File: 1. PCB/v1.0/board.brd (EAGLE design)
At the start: 69.5 x 114 mm, 2 parts

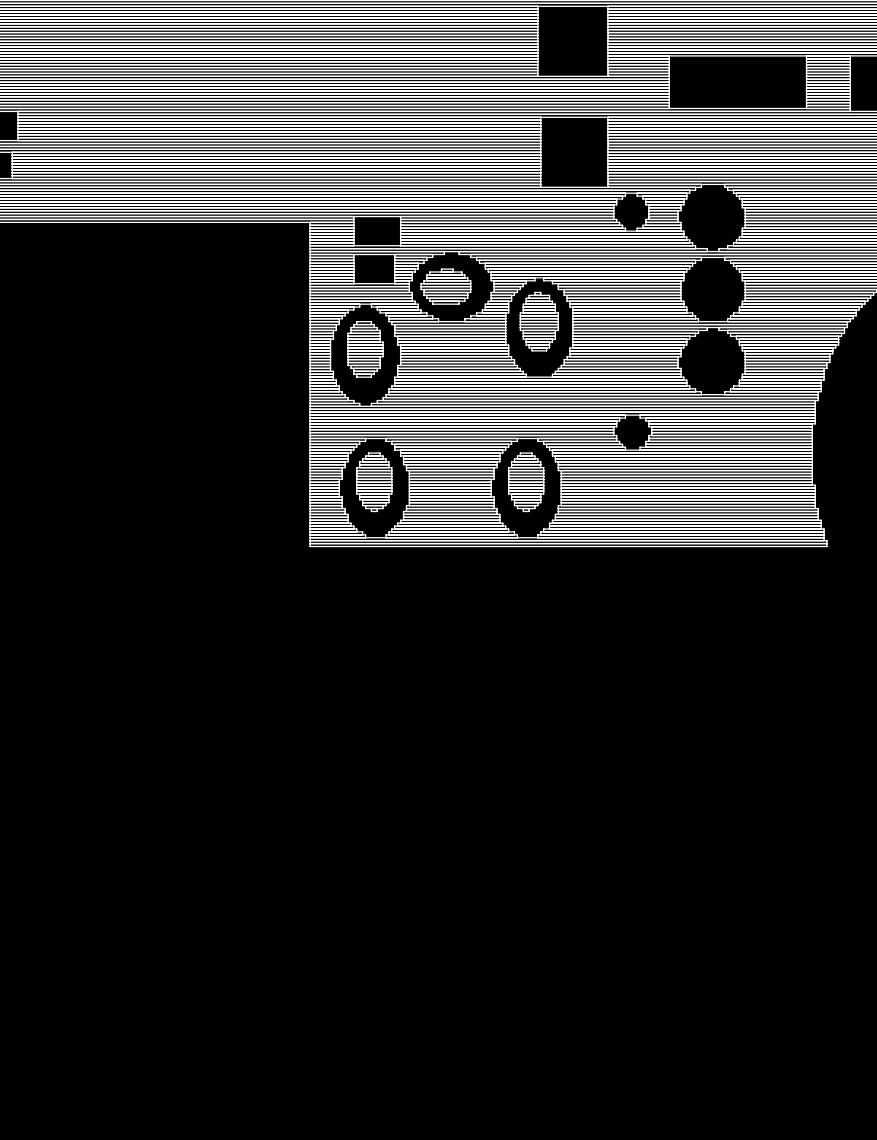
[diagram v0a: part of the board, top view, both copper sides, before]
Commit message: no message
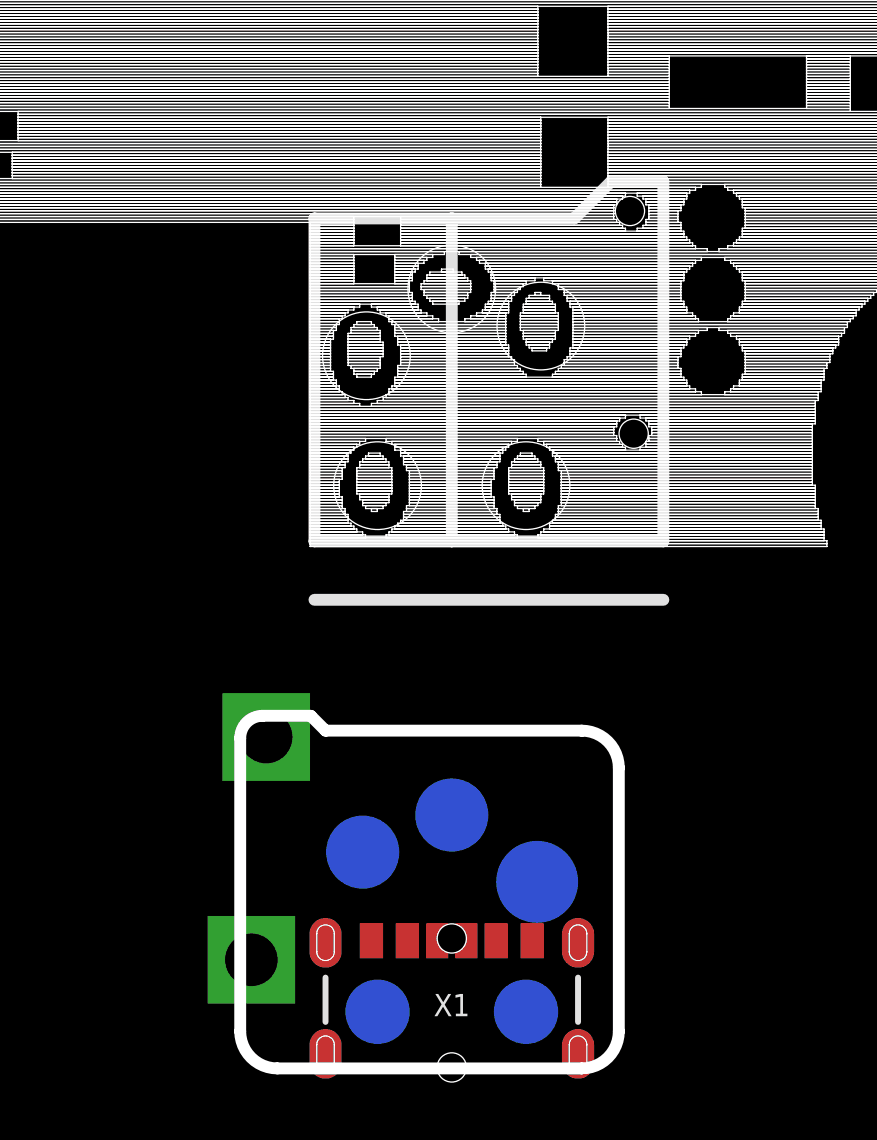
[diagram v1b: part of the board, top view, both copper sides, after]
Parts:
- added U$1: GBP_POWER_JACK, ,giltesa:GBP_POWER_JACK
- added X1: (no value), ,giltesa:USB-C_6P
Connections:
- new net VCC: U$1.VCC
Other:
- board size 69.5 x 114 mm -> 69.5 x 131.9 mm
